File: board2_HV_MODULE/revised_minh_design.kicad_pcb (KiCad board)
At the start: 2 copper layers, 100 x 42.2 mm, 13 parts, among them J1 Conn_01x07_Male, U1 LM7805_TO220, U2 NE5532, U3 CB101

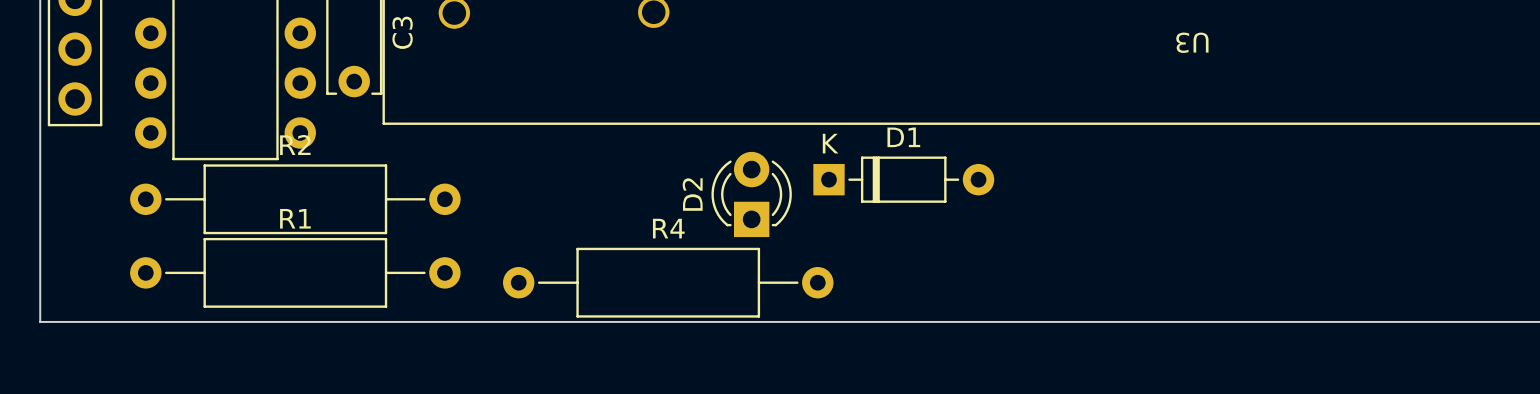
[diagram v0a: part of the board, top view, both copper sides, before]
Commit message: -
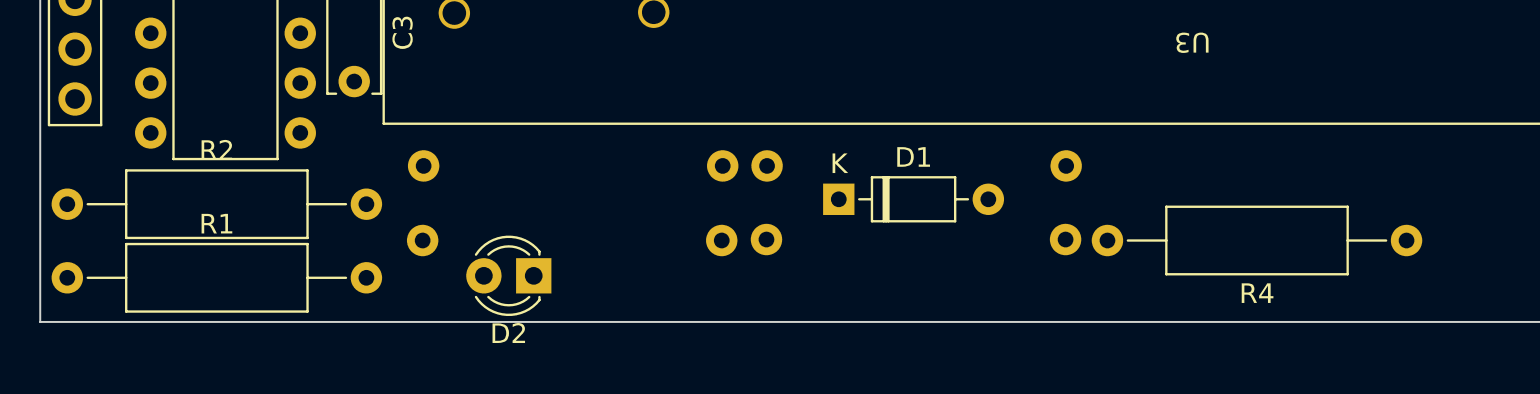
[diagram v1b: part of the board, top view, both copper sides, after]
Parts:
- added R5: 2K, Resistor_THT:R_Axial_DIN0309_L9.0mm_D3.2mm_P15.24mm_Horizontal, B.Cu at (120.8, 55.3)
- added R6: 1.1K, Resistor_THT:R_Axial_DIN0309_L9.0mm_D3.2mm_P15.24mm_Horizontal, B.Cu at (138.3, 55.3)
- added R7: 2K, Resistor_THT:R_Axial_DIN0309_L9.0mm_D3.2mm_P15.24mm_Horizontal, B.Cu at (120.7, 59.1)
- added R8: 1.1K, Resistor_THT:R_Axial_DIN0309_L9.0mm_D3.2mm_P15.24mm_Horizontal, B.Cu at (138.2, 59.0)
- moved R4 45.3 mm to (155.6, 59.1), turned to 180 degrees
- moved D2 11.5 mm to (111.1, 60.9), turned to 180 degrees
- moved R1 4.01 mm to (87.4, 61.0)
- moved R2 4.01 mm to (87.4, 57.2)
- moved D1 1.12 mm to (126.7, 57.0)
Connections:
- J1 pad 4: VMON -> VMON_3V3
- J1 pad 5: IMON -> IMON_3V3
